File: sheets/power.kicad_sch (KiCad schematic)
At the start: 79 parts, among them Q11 C1815, Q12 A1015, Q13 A1442, T1 COIL, U11 74LS05, U12 74LS06, U28 PC4741, U29 PC4741, U33 74AS04, U37 LM2576T-5, U38 74HC32, U8 74HC04, U80 74HC04

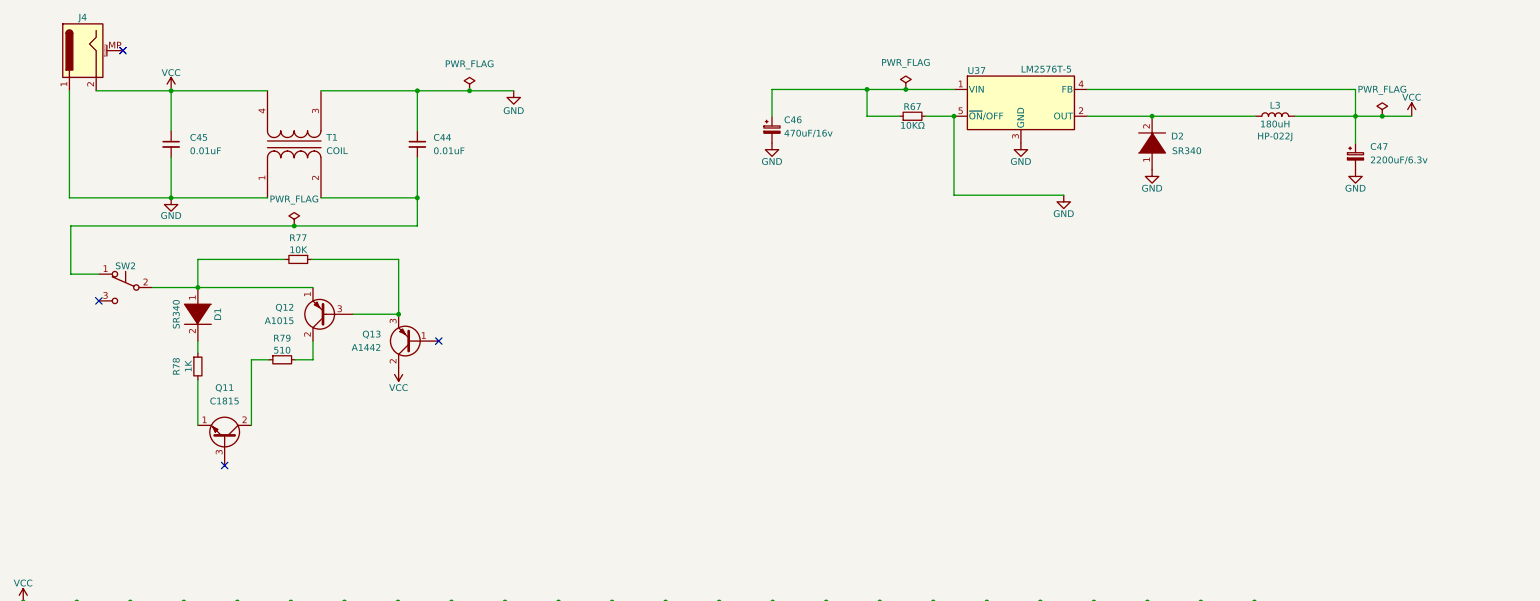
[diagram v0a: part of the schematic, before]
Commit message: Update Power Circuit 4
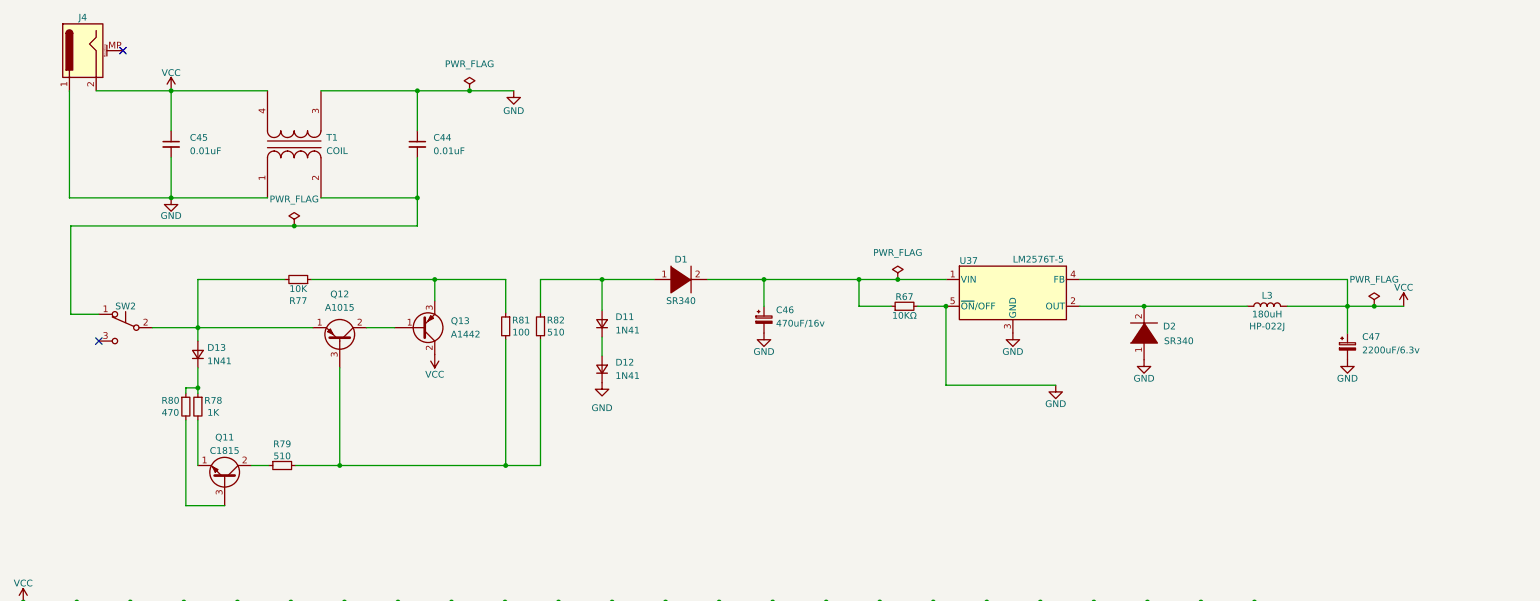
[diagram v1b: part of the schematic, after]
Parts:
- added D11, D12, D13: 1N41, symbol Device:D_Small
- added R80: 470, 1_NeoGeoLibrary:CAP3-5mm, symbol Device:R_Small
- added R81: 100, 1_NeoGeoLibrary:CAP3-5mm, symbol Device:R_Small
- added R82: 510, 1_NeoGeoLibrary:CAP3-5mm, symbol Device:R_Small
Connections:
- net GND: now also D12.1 (K)
- net at C46.1, R67.1, U37.1 (VIN): now also D1.2 (A)
- net at Q13.1 (B): now also Q12.2 (C)
- net at Q13.3 (E), R77.1: now also R81.1; no longer Q12.3 (B)
- net at Q12.1 (E), R77.2, SW2.2 (B): now also D13.2 (A); no longer D1.1 (K)
- net at R79.2: now also Q12.3 (B), R81.2, R82.2; no longer Q12.2 (C)
- net at Q11.3 (B): now also R80.2
- net at R78.1: now also D13.1 (K), R80.1; no longer D1.2 (A)
- new net: D11.1 (K), D12.2 (A)
- new net: D1.1 (K), D11.2 (A), R82.1
- no-connect marks 13 -> 11
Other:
- moved on the sheet: C46, C47, D1, D2, L3, Q11, Q12, Q13, R67, R77, R78, R79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

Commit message: Update Power Circuit 5
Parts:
- D11, D12, D13: footprint (none) -> Diode_THT:D_A-405_P10.16mm_Horizontal
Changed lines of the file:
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@@
       (effects (font (size 1.27 1.27)) (justify right))
     )
-    (property "Footprint" "" (id 2) (at 128.27 82.804 90)
+    (property "Footprint" "Diode_THT:D_A-405_P10.16mm_Horizontal" (id 2) (at 128.27 82.804 90)
       (effects (font (size 1.27 1.27)) hide)
     )
@@
       (effects (font (size 1.27 1.27)) (justify right))
     )
-    (property "Footprint" "" (id 2) (at 51.562 80.01 90)
+    (property "Footprint" "Diode_THT:D_A-405_P10.16mm_Horizontal" (id 2) (at 51.562 80.01 90)
       (effects (font (size 1.27 1.27)) hide)
     )
@@
       (effects (font (size 1.27 1.27)) (justify right))
     )
-    (property "Footprint" "" (id 2) (at 128.27 74.168 90)
-      (effects (font (size 1.27 1.27)) hide)
-    )
+    (property "Footprint" "Diode_THT:D_A-405_P10.16mm_Horizontal" (id 2) (at 128.27 74.168 90)
+      (effects (font (size 1.27 1.27)) hide)
+    )

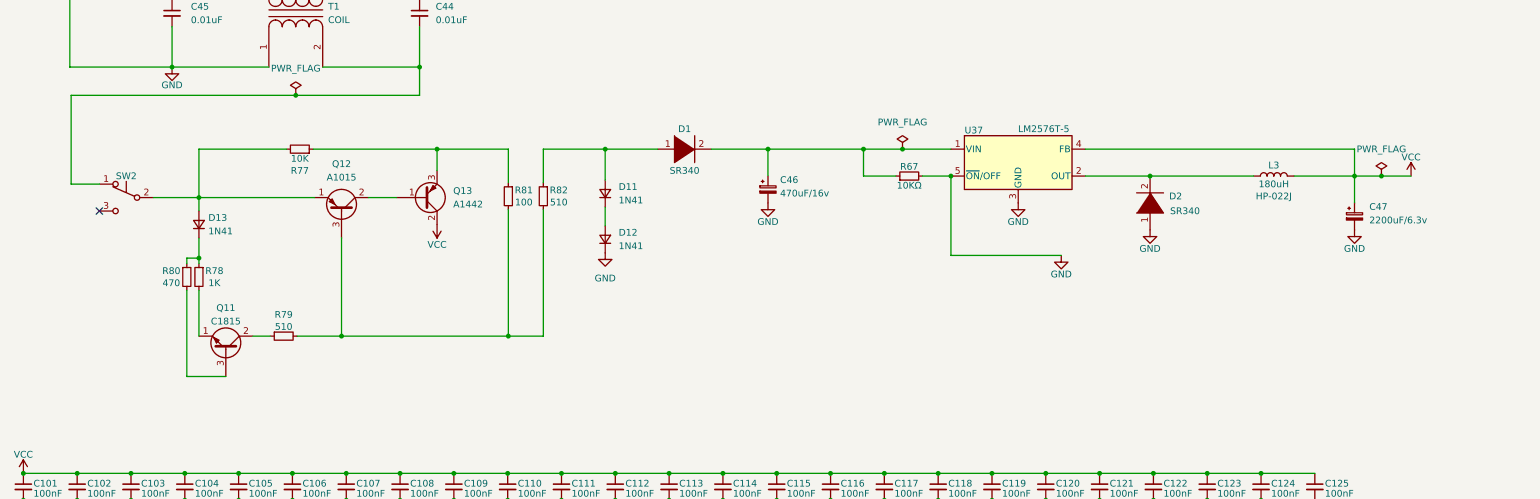
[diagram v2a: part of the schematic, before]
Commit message: Power Circuit Update 6
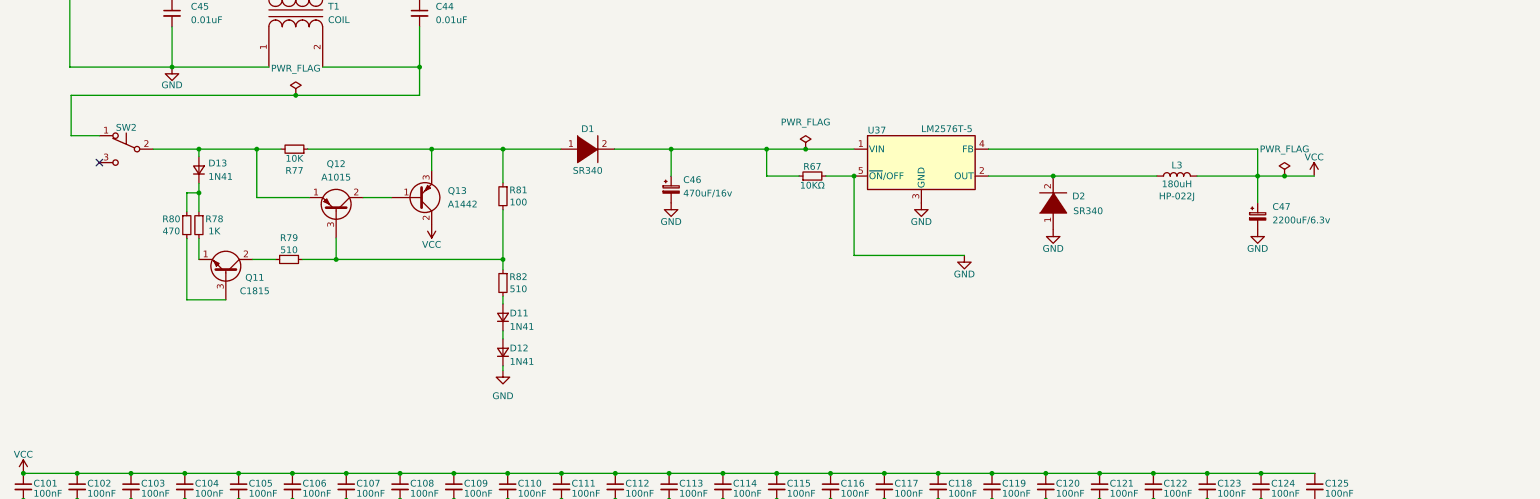
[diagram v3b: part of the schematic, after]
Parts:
- SW2: footprint (none) -> Button_Switch_THT:SW_Slide_1P2T_CK_OS102011MS2Q
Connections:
- net at Q13.3 (E), R77.1, R81.1: now also D1.1 (K)
- net at Q12.3 (B), R79.2, R81.2: now also R82.1; no longer R82.2
- new net: D11.2 (A), R82.2
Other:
- moved on the sheet: C46, C47, D1, D11, D12, D13, D2, L3, Q11, Q12, Q13, R67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

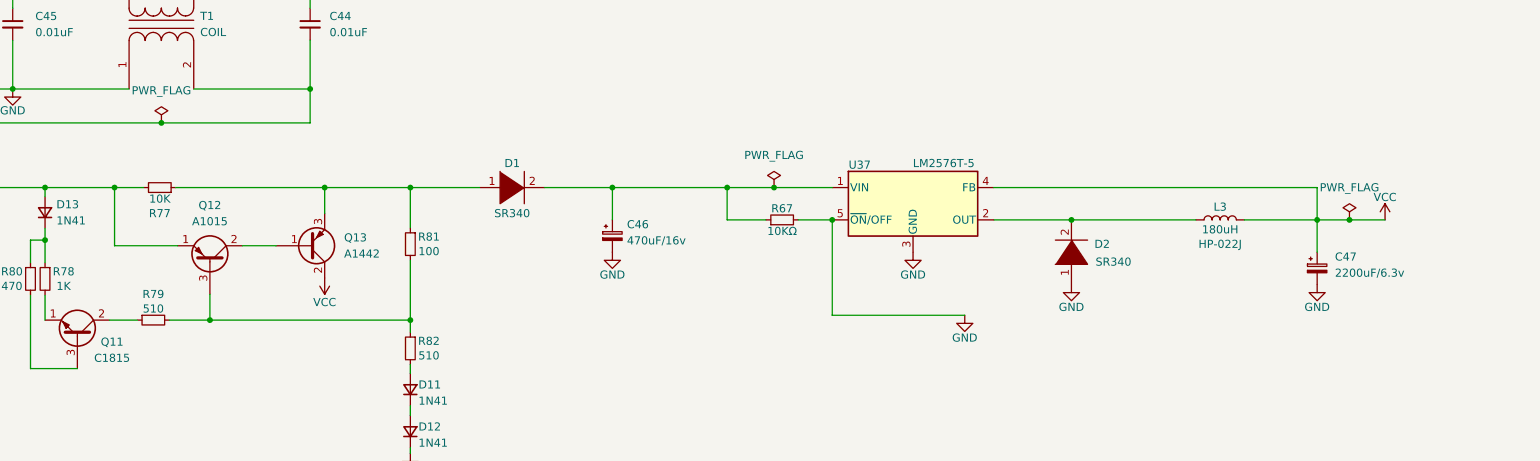
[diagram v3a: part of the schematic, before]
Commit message: Update Power Circuit 7
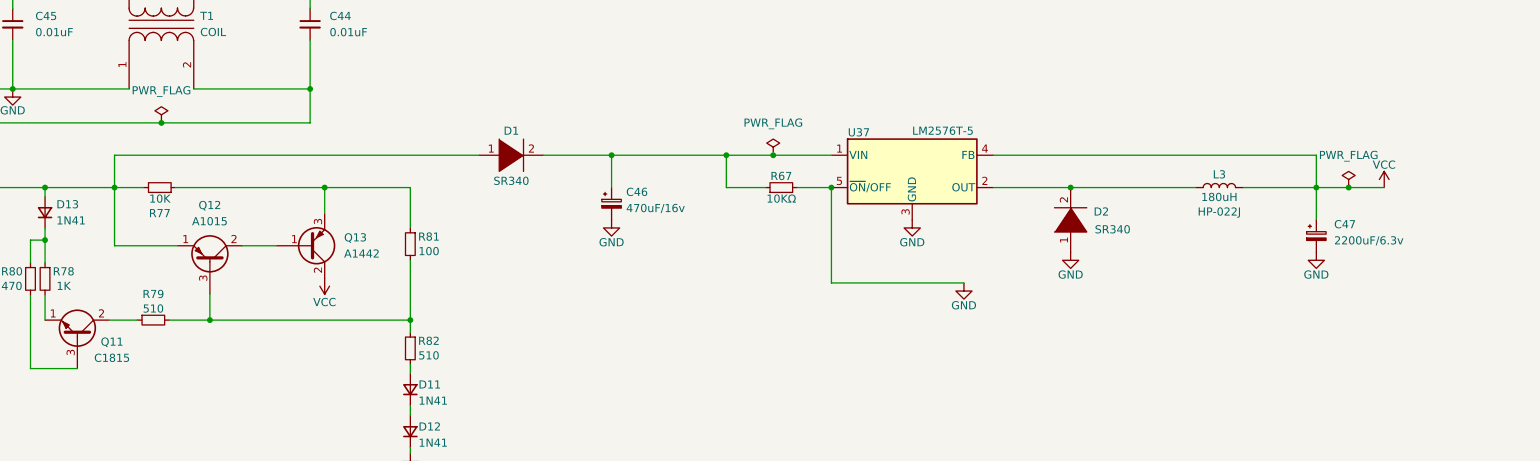
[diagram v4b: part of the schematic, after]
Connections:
- net at Q13.3 (E), R77.1, R81.1: no longer D1.1 (K)
- net at D13.2 (A), Q12.1 (E), R77.2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: now also D1.1 (K)
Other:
- moved on the sheet: C46, C47, D1, D2, L3, R67, U37
